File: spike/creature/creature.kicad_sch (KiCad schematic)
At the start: 72 parts, among them CN1 SWD PINS, CN16 HP OUT, CN2 SAO connector, J1 Conn_01x32, SW1 K3-1296S-E1_C128955, SW2 RST, U0 ATtiny1616-M, U1 ATtiny1616-M, U2 ATtiny1616-M, U3 ATSAMD21G18A-M, U4 AP2112K-3.3, U5 H3V3U10B, U6 LM4853MM/NOPB, U7 H3V3U10B, X2 Q13FC1350000400

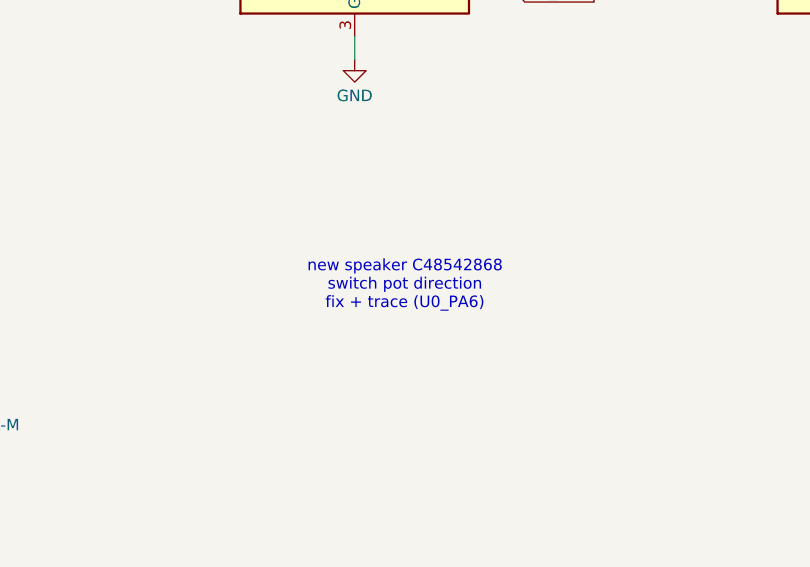
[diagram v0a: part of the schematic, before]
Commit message: yes
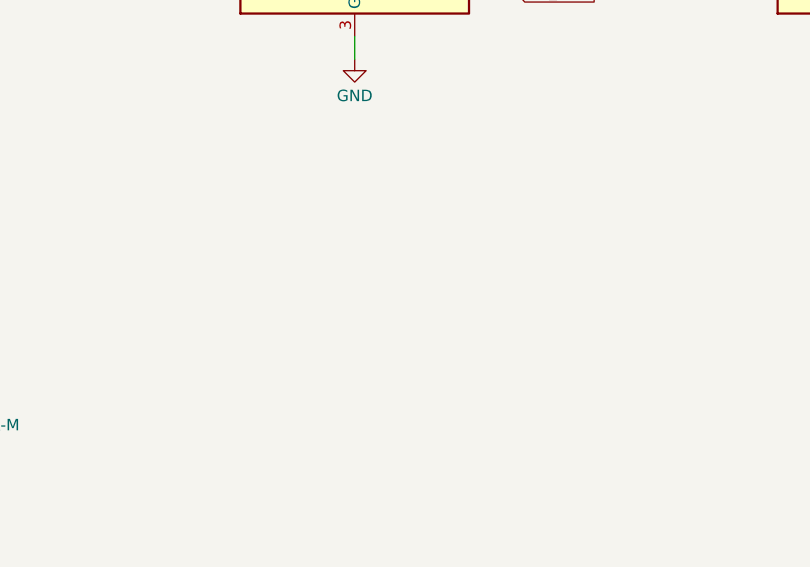
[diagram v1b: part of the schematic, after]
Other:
- note removed: "new speaker C48542868 switch pot direction fix + trace (U0_PA6)"
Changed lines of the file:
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@@
-		)
-	)
-	(text "new speaker C48542868\nswitch pot direction\nfix + trace (U0_PA6)"
-		(exclude_from_sim no)
-		(at 145.288 169.926 0)
-		(effects
-			(font
-				(size 1.27 1.27)
-			)
 		)
 	)

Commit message: madde
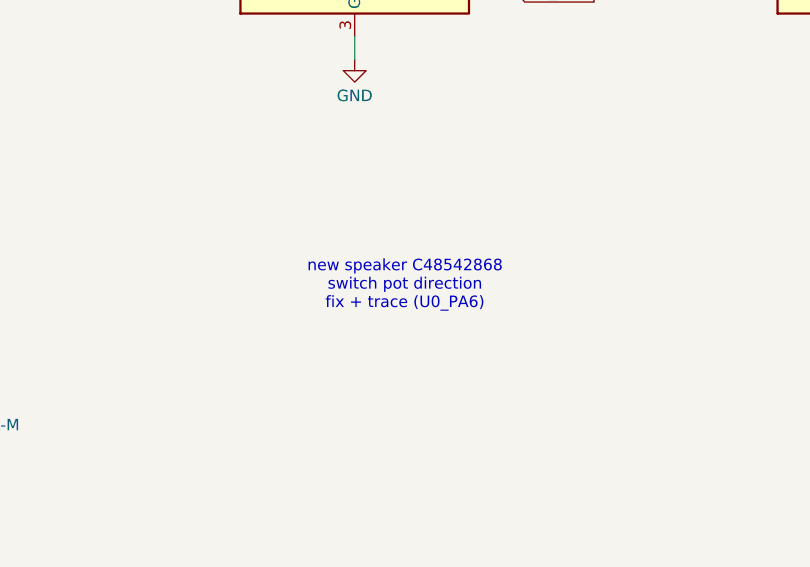
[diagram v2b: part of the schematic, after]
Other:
- note added: "new speaker C48542868 switch pot direction fix + trace (U0_PA6)"
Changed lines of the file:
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@@
+		)
+	)
+	(text "new speaker C48542868\nswitch pot direction\nfix + trace (U0_PA6)"
+		(exclude_from_sim no)
+		(at 145.288 169.926 0)
+		(effects
+			(font
+				(size 1.27 1.27)
+			)
 		)
 	)
